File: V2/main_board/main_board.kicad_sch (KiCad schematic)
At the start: 102 parts, among them J1 USB_C_Receptacle_USB2.0_16P, J2 OUT_1, J3 Conn_02x14_Top_Bottom, J4 OUT_2, J5 EXT_TEMP, K1 Relay_SPST_Latching_2coil, K2 Relay_SPST_Latching_2coil, Q1 2N7002, Q2 BC817, Q3 BC817, Q4 BC817, Q5 BC817, SW1 SW_Push, SW2 SW_Push, SW3 SW_SPDT, U1 SRV05-4, U10 MAX17048G_T10, U11 LTV-217, U12 DS18B20Z, U13 DS18B20Z, U14 LTV-217, U2 BQ24075RGT, U3 DW01A, U4 ESP32-S3-WROOM-2, U5 FS8205A, U6 LTV-217, U7 AP7361C-33E, U8 PCF8563T, U9 LTV-217, Y1 32.768khz

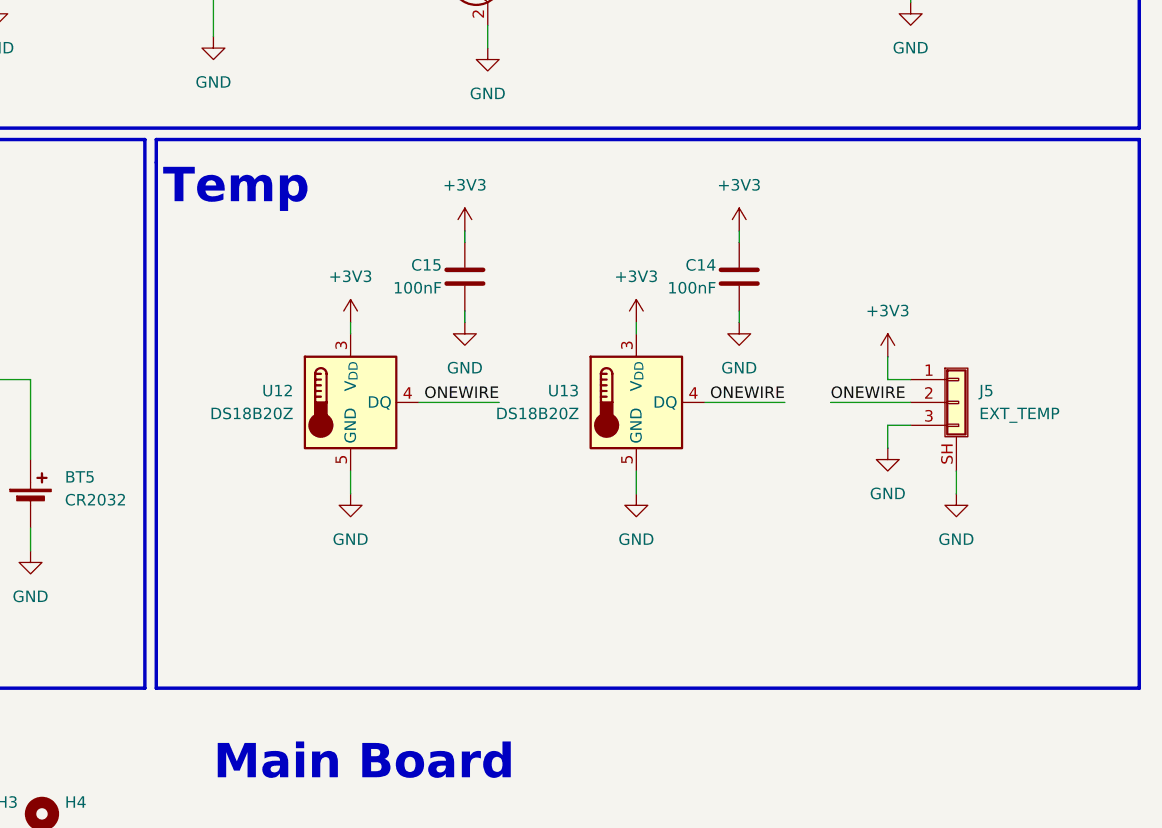
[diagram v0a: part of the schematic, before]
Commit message: fix symbol
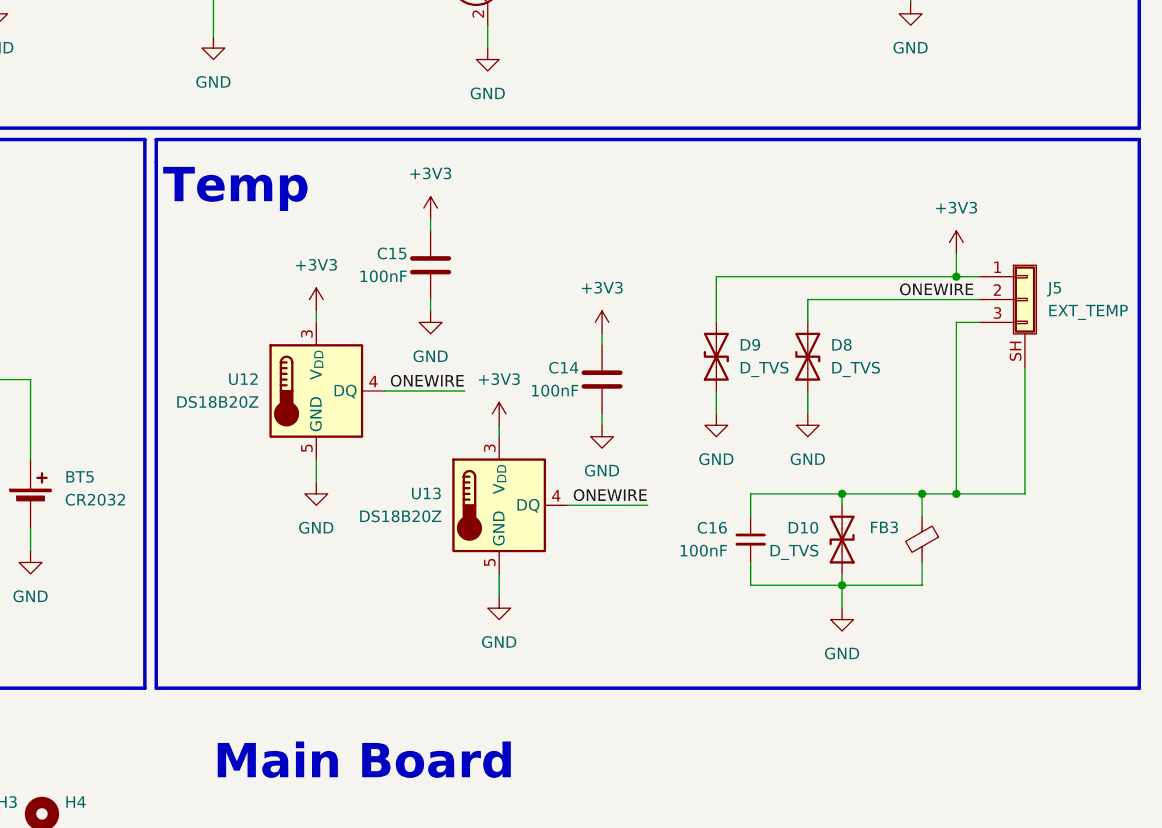
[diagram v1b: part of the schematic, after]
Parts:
- added C16: 100nF, Capacitor_SMD:C_0603_1608Metric, symbol *partsbox:0603-100nF
- added D10, D8, D9: D_TVS, Diode_SMD:D_SOD-323, symbol *partsbox:H8VHD3B
- added FB3: FerriteBead_Small, Inductor_SMD:L_0603_1608Metric, symbol *partsbox:BLM18PG121SN1D
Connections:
- net +3V3: now also D9.2 (A2)
- net GND: now also C16.2, D10.1 (A1), D8.1 (A1), D9.1 (A1), FB3.2; no longer J5.3 (Pin_3), J5.SH (Shield)
- net ONEWIRE: now also D8.2 (A2)
- new net: C16.1, D10.2 (A2), FB3.1, J5.3 (Pin_3), J5.SH (Shield)
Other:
- moved on the sheet: C14, C15, J5, U12, U13
